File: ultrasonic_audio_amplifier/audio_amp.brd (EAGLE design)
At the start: 65 x 30 mm, 23 parts, among them CON1 MOLEX_5566-2, J1 282834-2, J2 282834-2, J3 MKDS_5/2-6,352, U1 DS1881Z-050+, U2 LM384_AUDIO_POWER_AMP

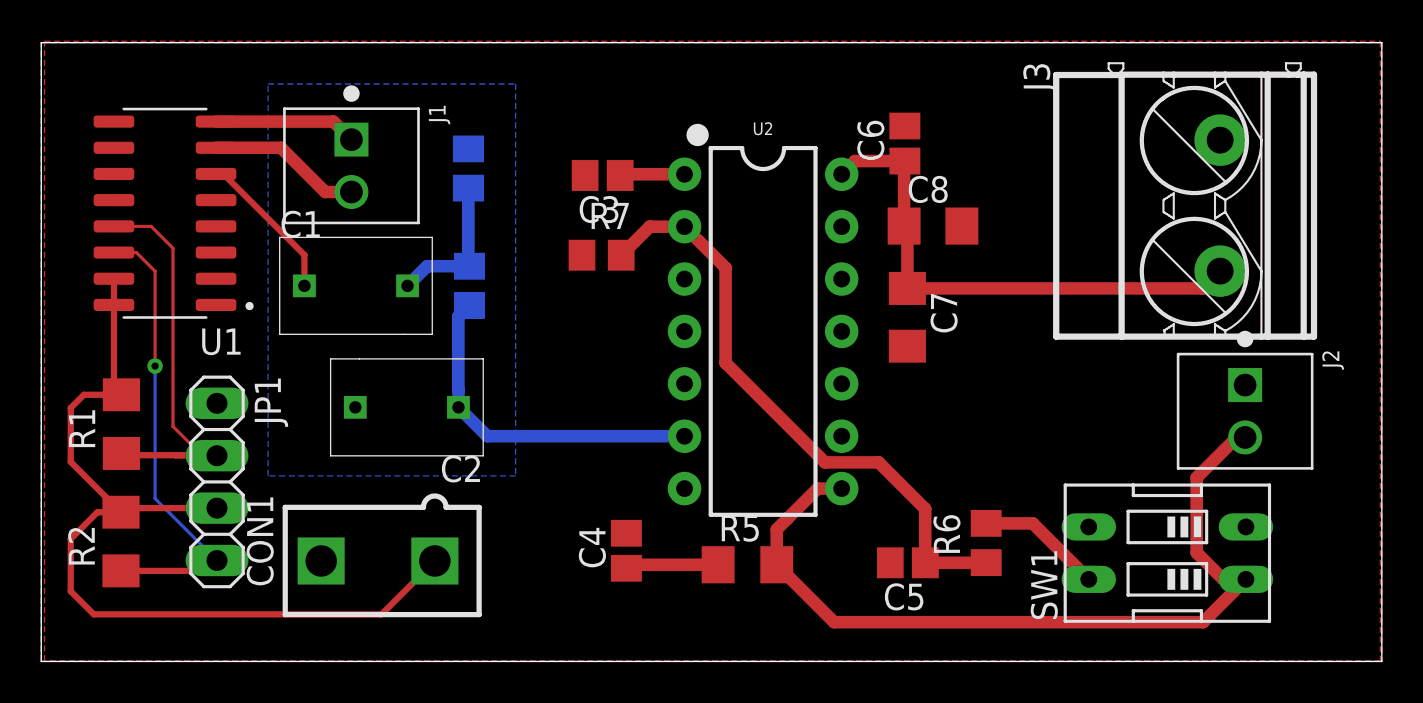
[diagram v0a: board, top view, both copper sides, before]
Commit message: Updated board layout for review
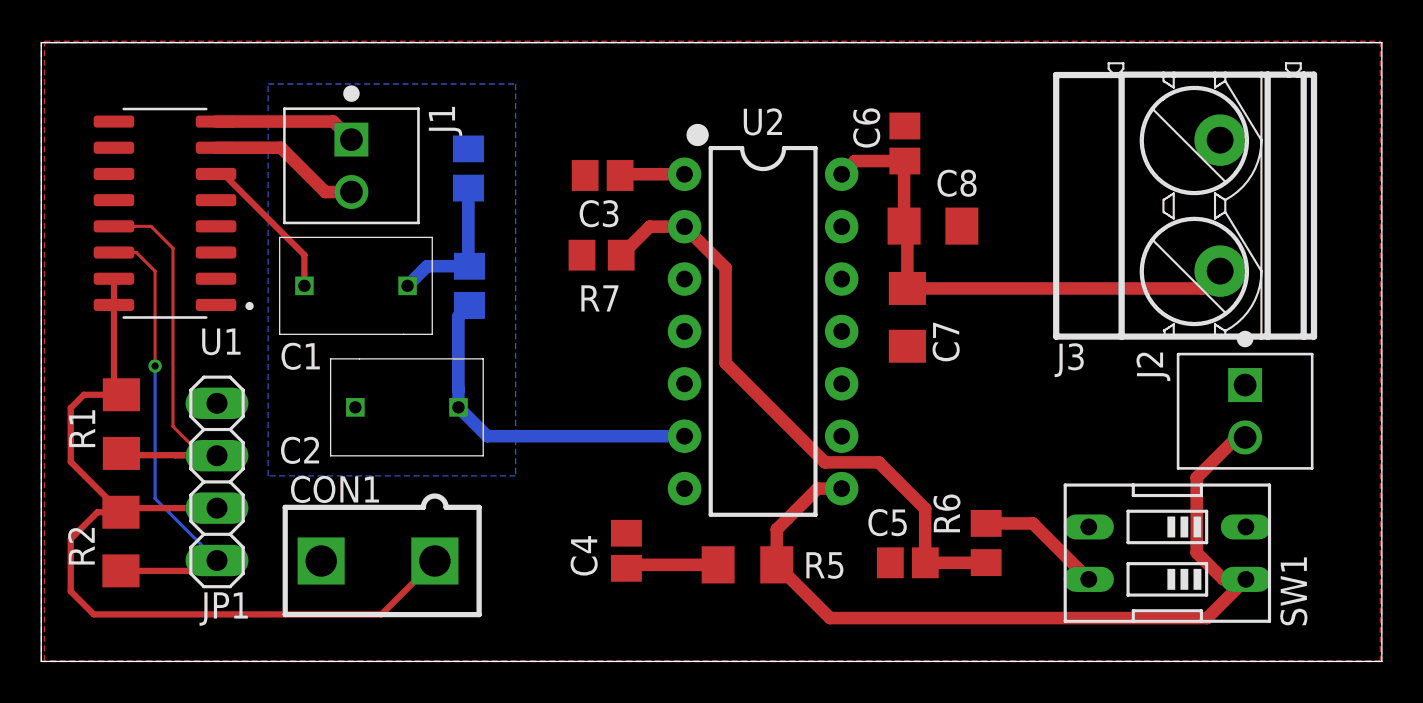
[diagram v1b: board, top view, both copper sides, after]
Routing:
- net SCL: track 24.1 -> 22.5 mm
- net SDA: track 21.0 -> 19.9 mm
